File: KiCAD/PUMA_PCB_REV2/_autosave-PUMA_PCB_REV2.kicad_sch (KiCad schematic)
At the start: 9 parts, among them J1 87832-0411, U1 MICROFC-30035-SMT-TR1, U2 MICROFC-30035-SMT-TR1

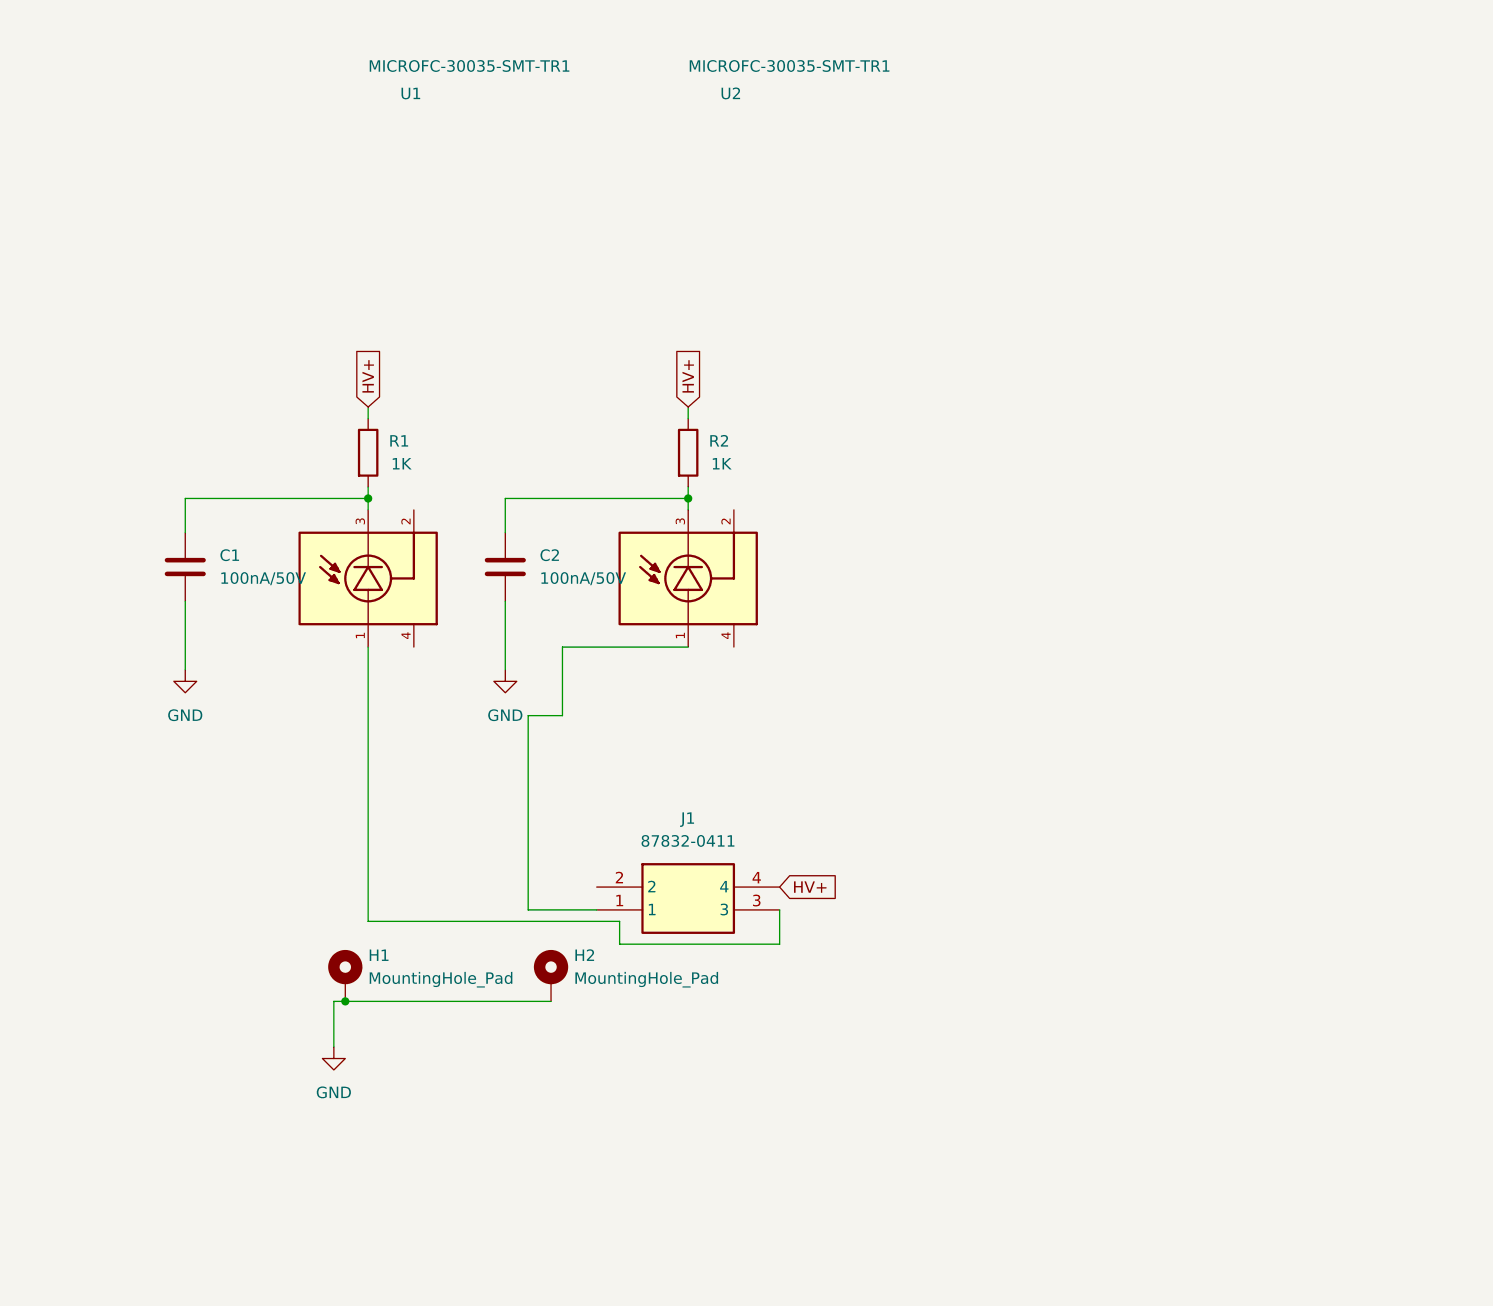
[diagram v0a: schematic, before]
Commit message: symmetric board iteration 1.0
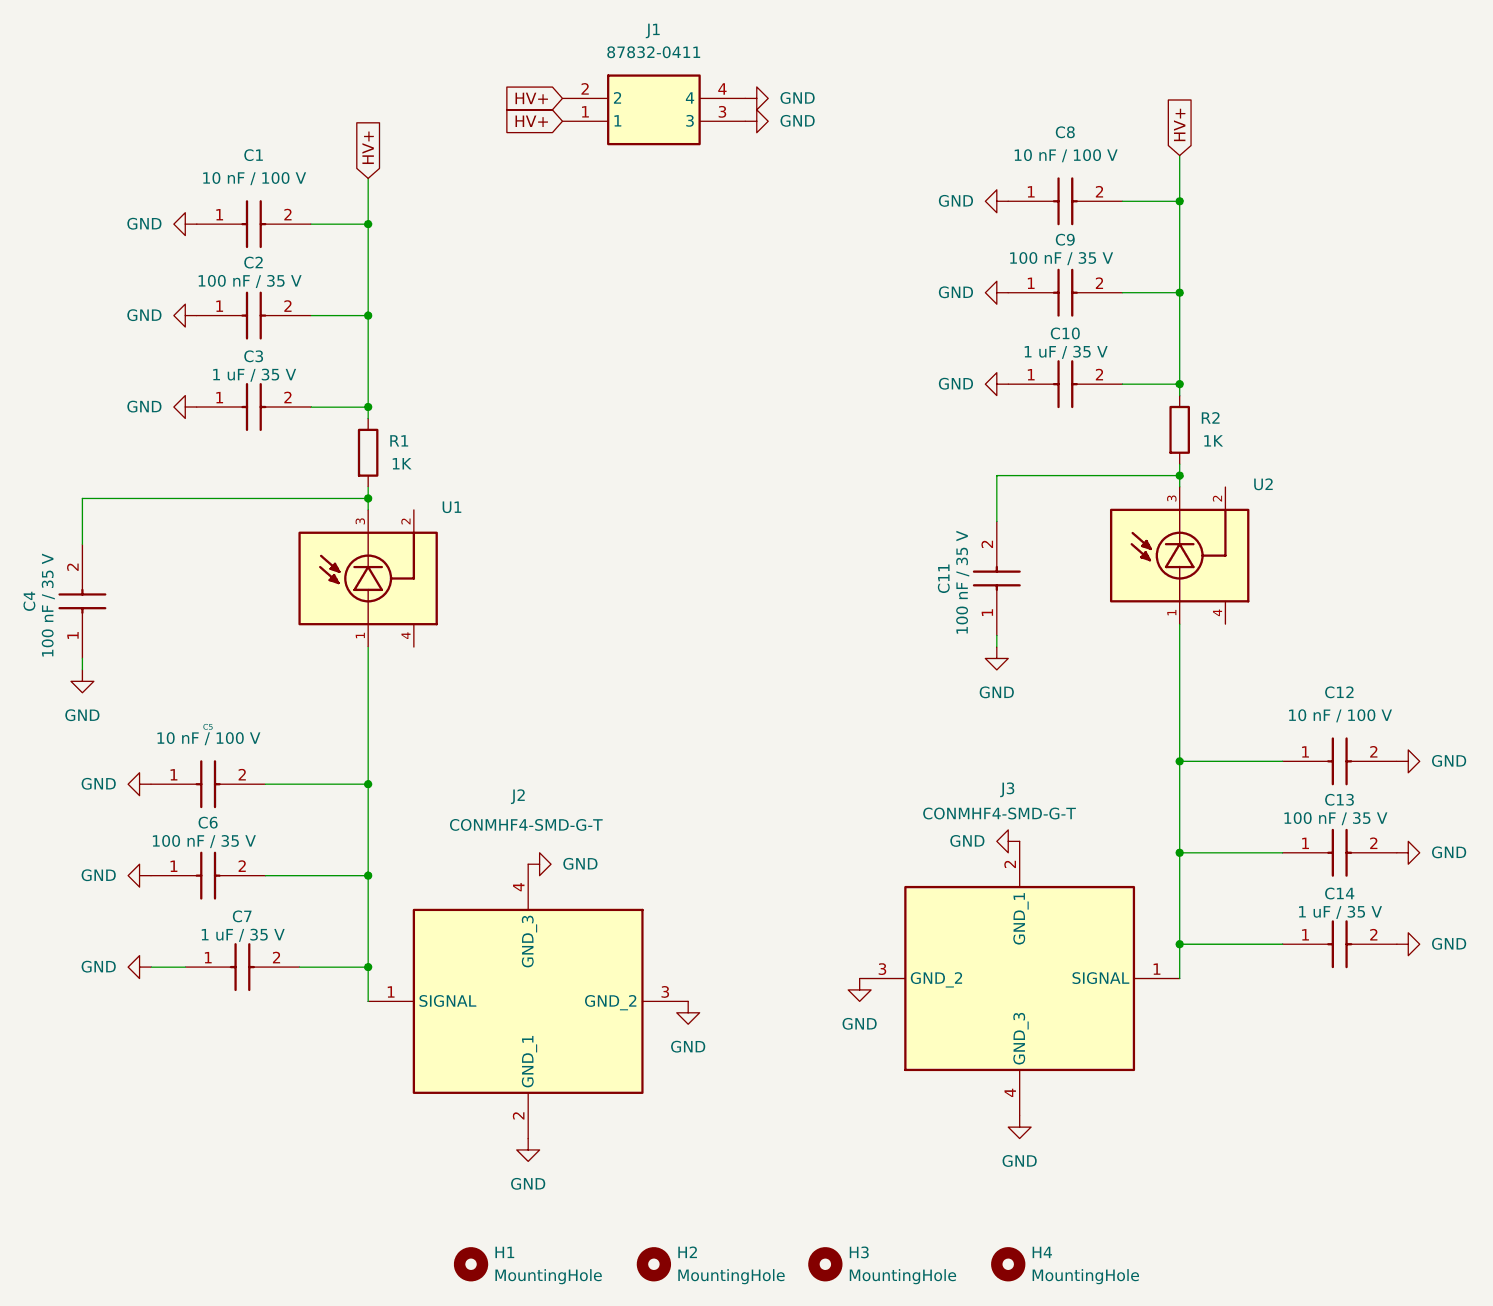
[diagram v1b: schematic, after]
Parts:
- removed C1, C2: 100nA/50V, Capacitor_SMD:C_1206_3216Metric, symbol Device:C
- removed H1, H2: MountingHole_Pad, MountingHole:MountingHole_2.5mm_Pad, symbol Mechanical:MountingHole_Pad
- added C1, C12, C5, C8: 10 nF / 100 V, SiPM_Onsemi:CAPC1608X90N_001uF, symbol CGA3EANP02A103J080AC_001uF:CGA3EANP02A103J080AC
- added C10, C14, C3, C7: 1 uF / 35 V, SiPM_Onsemi:CAPC1608X90N_1uF, symbol MMJCG168CB7105KRPA18_1uF:MMJCG168CB7105KRPA18
- added C11, C13, C2, C4, C6, C9: 100 nF / 35 V, SiPM_Onsemi:CAPC1608X90N_1uF, symbol CGA3EANP02A103J080AC_001uF:CGA3EANP02A103J080AC
- added H1, H2: MountingHole, MountingHole:CastellatedHole, symbol Mechanical:MountingHole
- added H3, H4: MountingHole, MountingHole:Castelated_Hold_Right, symbol Mechanical:MountingHole
- added J2, J3: CONMHF4-SMD-G-T, SiPM_Onsemi:CONMHF4SMDGT, symbol CONMHF4-SMD-G-T:CONMHF4-SMD-G-T
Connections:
- net GND: now also J1.3, J1.4, C1.1, C10.1, C11.1, C12.2, C13.2, C14.2, C2.1, C3.1, C4.1, C5.1, C6.1, C7.1, C8.1, C9.1, J2.2 (GND_1), J2.3 (GND_2), J2.4 (GND_3), J3.2 (GND_1), J3.3 (GND_2), J3.4 (GND_3)
- net HV+: now also J1.1, J1.2, C1.2, C10.2, C2.2, C3.2, C8.2, C9.2; no longer J1.4
- net at R1.2, U1.3: now also C4.2
- net at R2.2, U2.3: now also C11.2
- net at U2.1: now also C12.1, C13.1, C14.1, J3.1 (SIGNAL); no longer J1.1
- net at U1.1: now also C5.2, C6.2, C7.2, J2.1 (SIGNAL); no longer J1.3
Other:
- moved on the sheet: J1
